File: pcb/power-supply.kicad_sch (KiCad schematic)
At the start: 23 parts, among them IC1 AP2112K-3.3TRG1, IC3 INA199B2, IC4 AP62300TWU-7

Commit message: added DIP switches, footprints
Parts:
- IC3: footprint (none) -> sc70:SC70-6L
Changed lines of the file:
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@@
       (effects (font (size 1.27 1.27)) (justify left bottom))
     )
-    (property "Footprint" "" (at 86.36 101.6 0)
+    (property "Footprint" "sc70:SC70-6L" (at 86.36 101.6 0)
       (effects (font (size 1.27 1.27)) hide)
     )

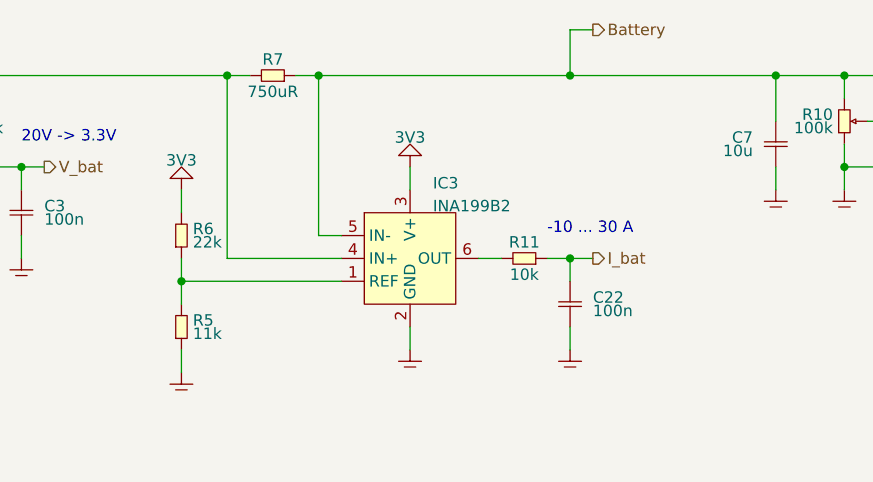
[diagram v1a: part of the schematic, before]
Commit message: updated components. worked on layout
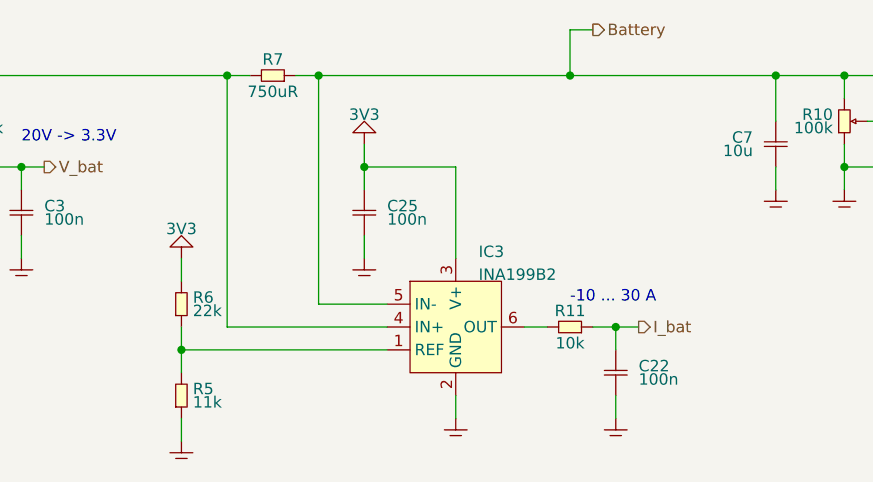
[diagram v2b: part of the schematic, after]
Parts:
- added C25: 100n, SMT:0603, symbol generic:C
- L1: footprint (none) -> inductor:5x5; DigiKey (none) -> 445-174398-1-ND; MPN (none) -> VLS5045EX-3R3N
- R7: footprint (none) -> SMT:2512-high-current
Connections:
- net 3V3: now also C25.1
- net GND: now also C25.2
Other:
- moved on the sheet: C22, IC3, R11, R5, R6
